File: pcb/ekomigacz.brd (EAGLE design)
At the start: 26.7 x 38.7 mm, 9 parts, among them X1 USB-A-H

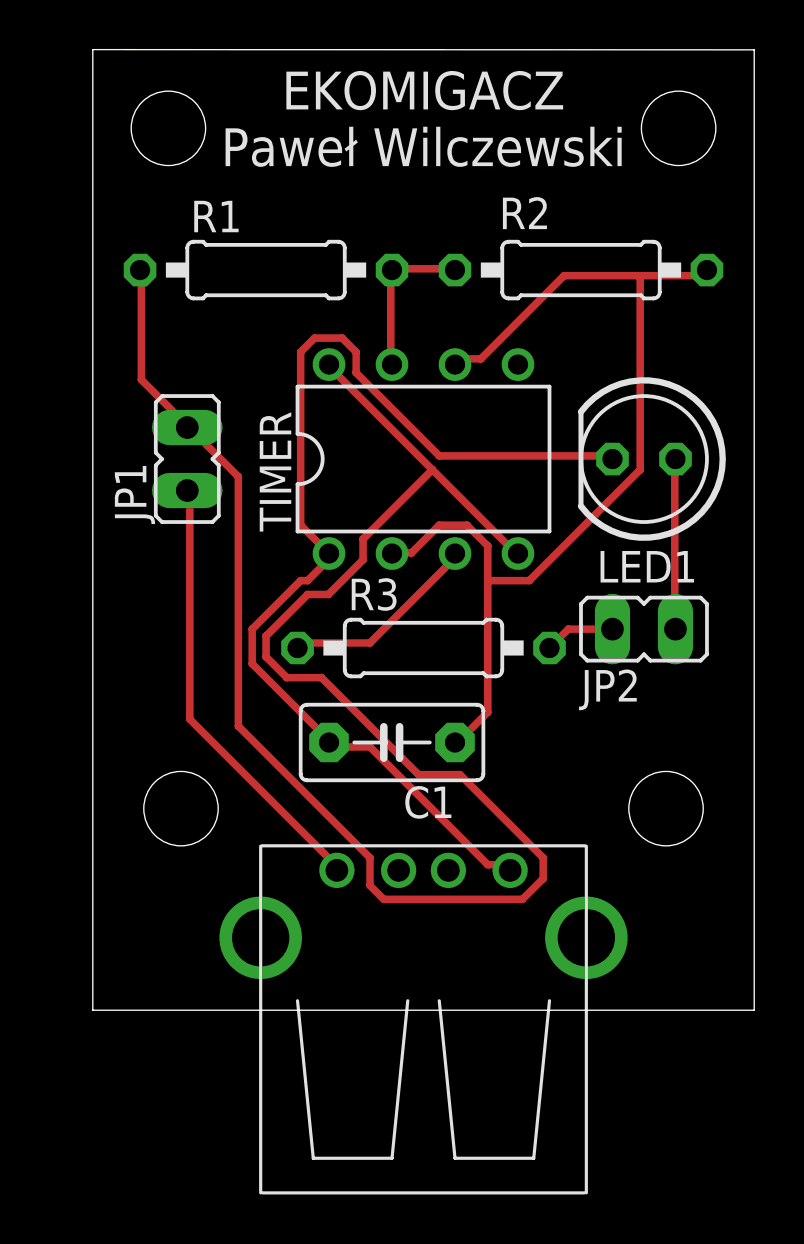
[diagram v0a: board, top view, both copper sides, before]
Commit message: PCB and model update
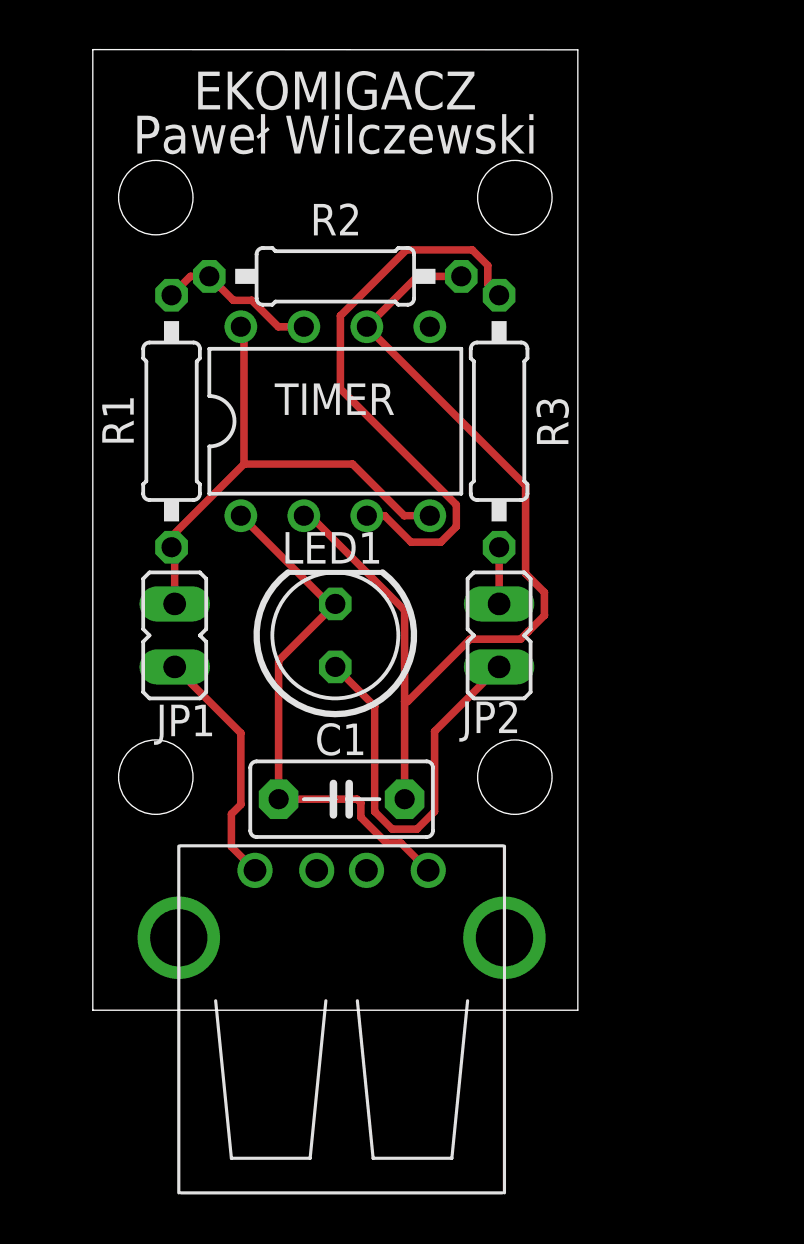
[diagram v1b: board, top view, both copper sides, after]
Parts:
- moved LED1 14.3 mm to (9.78, 15.1), turned to 90 degrees
- moved R2 9.91 mm to (9.78, 29.6)
- moved R3 9.64 mm to (16.4, 23.7), turned to 270 degrees
- moved R1 7.19 mm to (3.17, 23.7), turned to 90 degrees
- moved JP1 7.13 mm to (3.30, 15.1)
- moved JP2 5.85 mm to (16.4, 15.1), turned to 180 degrees
- moved TIMER 3.87 mm to (9.78, 23.7)
- moved X1 3.30 mm to (10.0, 2.92)
- moved C1 3.06 mm to (10.0, 8.51)
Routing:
- net N$4: track 73.2 -> 20.8 mm
- net N$9: track 43.8 -> 21.7 mm
- net 5V: track 8.04 -> 23.4 mm
- net N$7: track 6.86 -> 16.4 mm
- net N$1: track 17.9 -> 9.86 mm
- net N$5: track 40.8 -> 39.6 mm
- net N$6: track 2.86 -> 2.29 mm
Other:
- board size 26.7 x 38.7 mm -> 19.6 x 38.7 mm
